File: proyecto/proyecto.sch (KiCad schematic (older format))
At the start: 34 parts, among them SW1 SW_Push, SW2 SW_Push

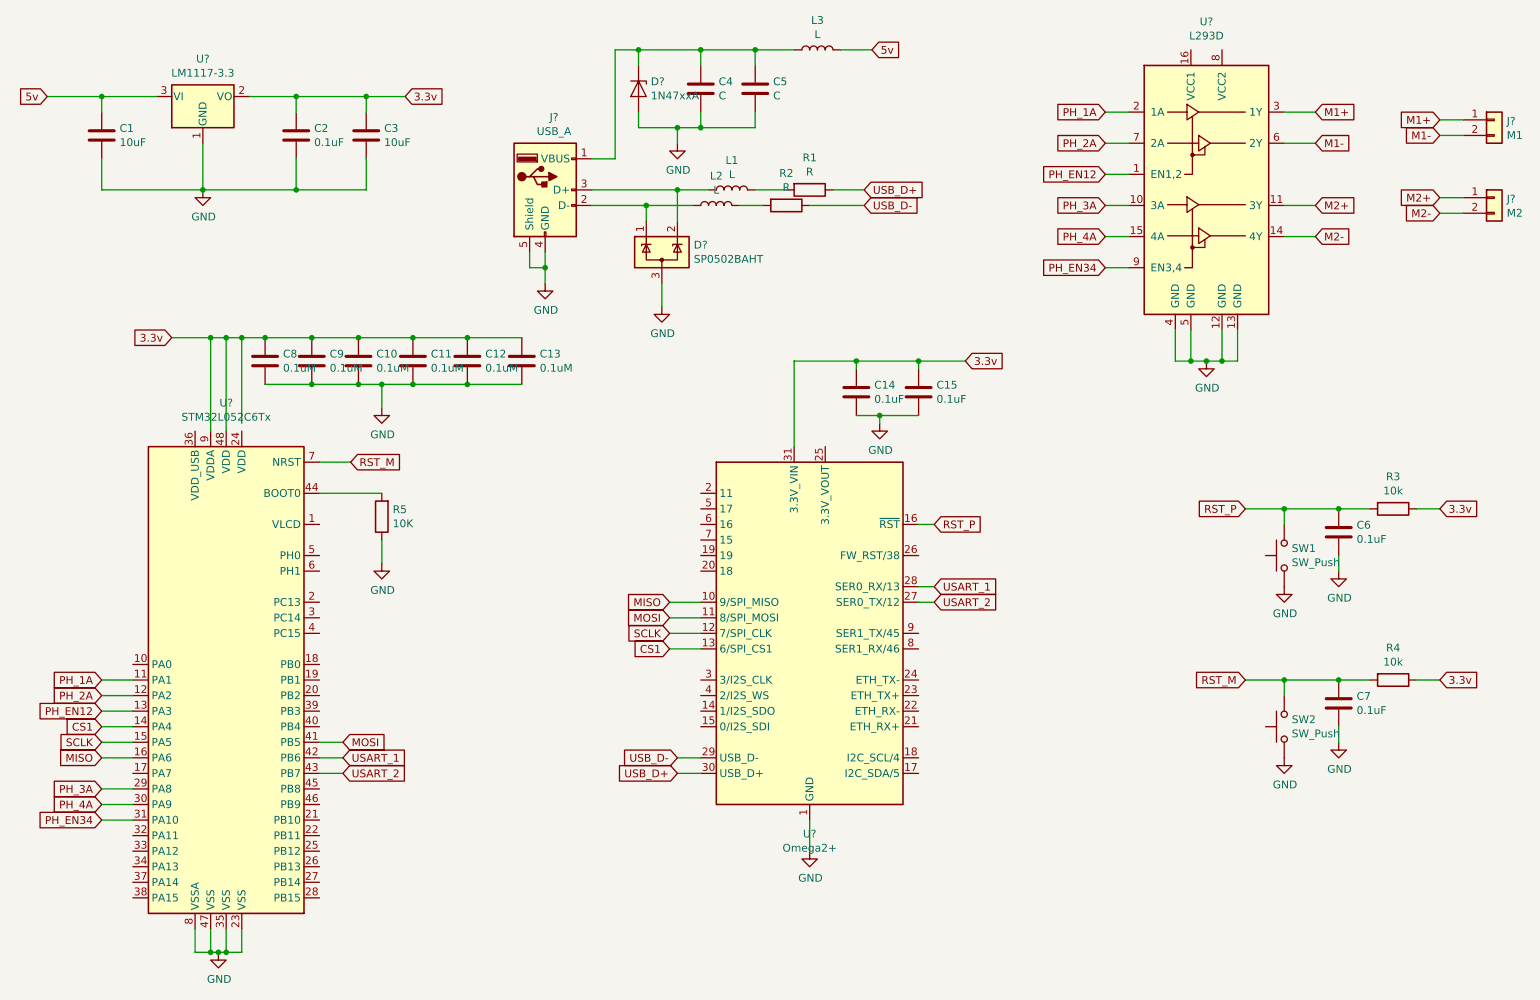
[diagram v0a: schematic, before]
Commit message: Add files via upload
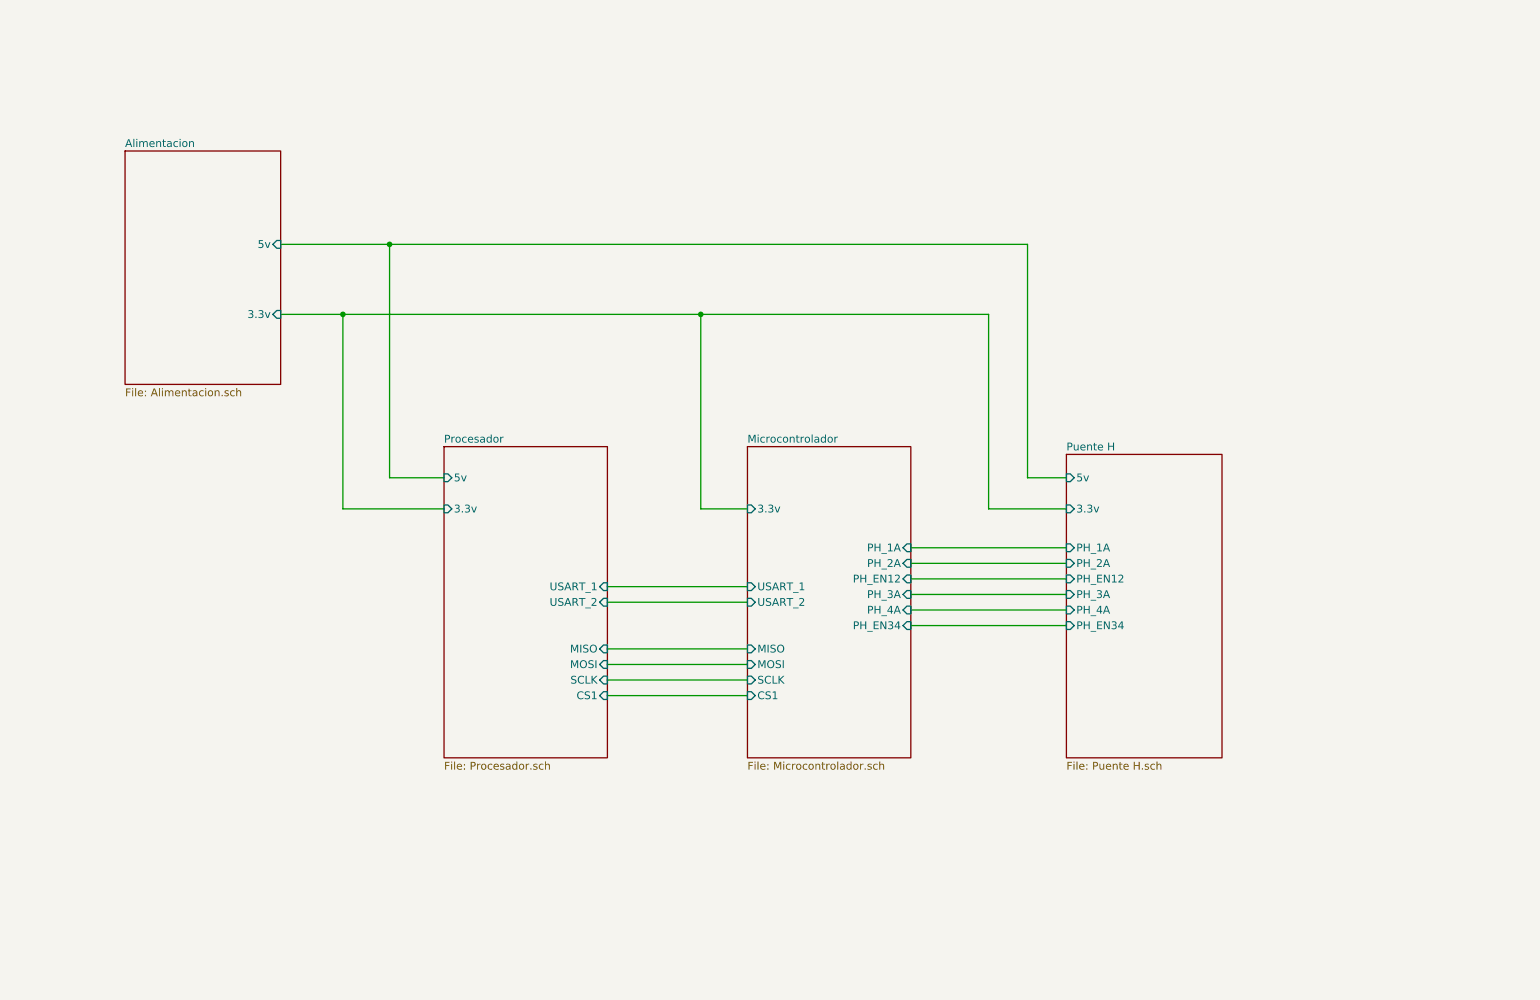
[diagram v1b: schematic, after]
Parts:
- removed C1, C3: 10uF, symbol Device:C
- removed C10, C11, C12, C13, C8, C9: 0.1uM, symbol Device:C
- removed C14, C15, C2, C6, C7: 0.1uF, symbol Device:C
- removed C4, C5: C, symbol Device:C
- removed D?: SP0502BAHT, Package_TO_SOT_SMD:SOT-23, symbol Power_Protection:SP0502BAHT
- removed D?: 1N47xxA, Diode_THT:D_DO-41_SOD81_P10.16mm_Horizontal, symbol Diode:1N47xxA
- removed J?: USB_A, symbol Connector:USB_A
- removed J?: M1, symbol Connector_Generic:Conn_01x02
- removed J?: M2, symbol Connector_Generic:Conn_01x02
- removed L1, L2, L3: L, symbol Device:L
- removed R1, R2: R, symbol Device:R
- removed R3, R4: 10k, symbol Device:R
- removed R5: 10K, symbol Device:R
- removed SW1, SW2: SW_Push, symbol Switch:SW_Push
- removed U?: Omega2+, Module:Onion_Omega2+, symbol MCU_Module:Omega2+
- removed U?: STM32L052C6Tx, Package_QFP:LQFP-48_7x7mm_P0.5mm, symbol MCU_ST_STM32L0:STM32L052C6Tx
- removed U?: L293D, Package_DIP:DIP-16_W7.62mm, symbol Driver_Motor:L293D
- removed U?: LM1117-3.3, symbol Regulator_Linear:LM1117-3.3
